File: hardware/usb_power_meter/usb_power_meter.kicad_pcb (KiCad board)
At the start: 4 copper layers, 33 x 24.6 mm, 30 parts, among them J1 Conn_ARM_JTAG_SWD_10, J2 USB_A, J4 USB_A, Q1 2N7002, Q2 IRML6401, U1 nRF52833-QDxx, U2 INA226, X1 32Mhz crystal, X2 32.768kHz crystal

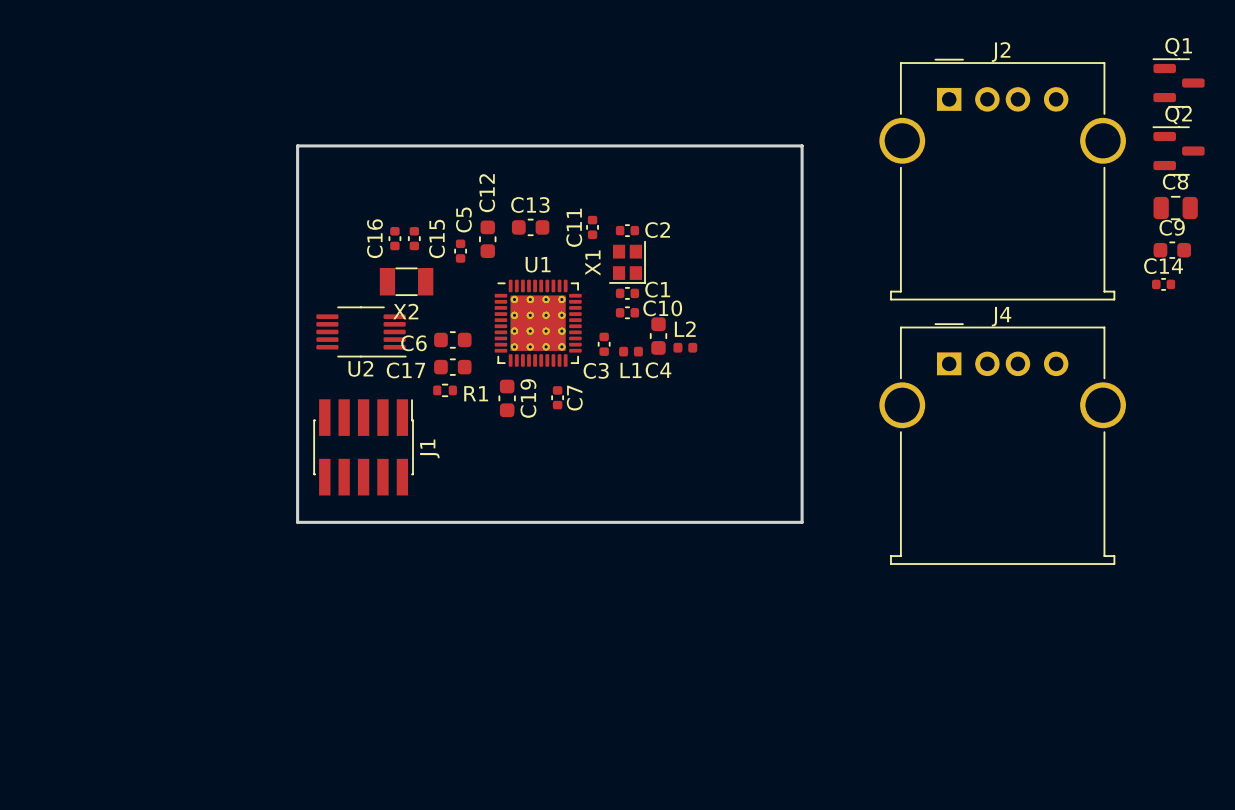
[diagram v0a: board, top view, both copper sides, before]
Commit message: Draft routing done
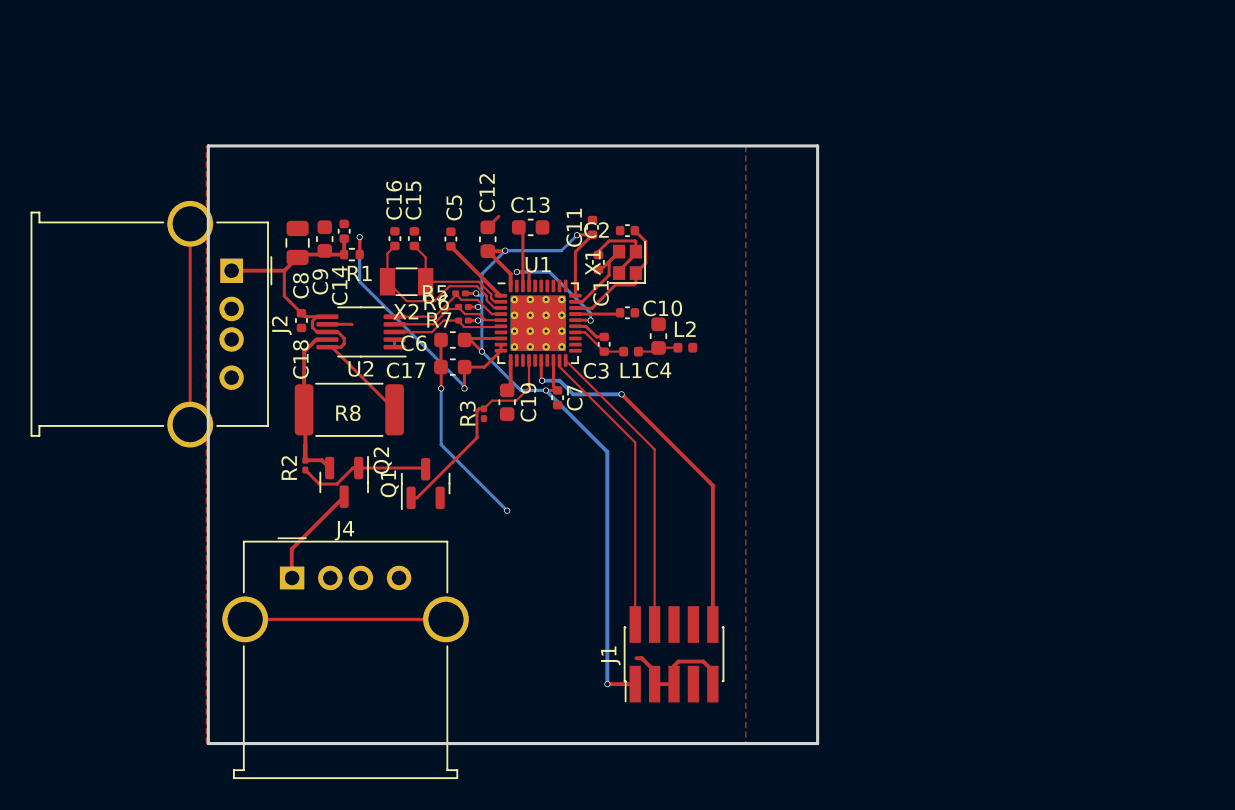
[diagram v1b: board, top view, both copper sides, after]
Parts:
- added C18: 100 nF, Capacitor_SMD:C_0402_1005Metric, F.Cu at (118.6, 102.6)
- added R2: 10k, Resistor_SMD:R_0201_0603Metric, F.Cu at (118.9, 112.1)
- added R3: 10k, Resistor_SMD:R_0201_0603Metric, F.Cu at (130.6, 108.7)
- added R5: 10k, Resistor_SMD:R_0201_0603Metric, F.Cu at (129.0, 100.8)
- added R6: 10k, Resistor_SMD:R_0201_0603Metric, F.Cu at (129.2, 101.7)
- added R7: 10k, Resistor_SMD:R_0201_0603Metric, F.Cu at (129.2, 102.6)
- added R8: LRP12FTDSR020, Resistor_SMD:R_2512_6332Metric, F.Cu at (121.8, 108.5)
- moved Q2 58.8 mm to (121.4, 113.2), turned to -90 degrees
- moved C8 57.5 mm to (118.4, 97.5), turned to 90 degrees
- moved Q1 55.8 mm to (126.7, 113.3), turned to 90 degrees
- moved C9 55.5 mm to (120.1, 97.3), turned to 90 degrees
- moved C14 53.7 mm to (121.4, 96.8), turned to 90 degrees
- moved J2 48.3 mm to (114.0, 99.4), turned to -90 degrees
- moved J4 45.2 mm to (118.0, 119.5)
- moved J1 24.4 mm to (143.0, 124.5), turned to 90 degrees
- moved R1 10.8 mm to (121.9, 98.3)
- moved C1 2.79 mm to (138.0, 98.8), turned to -90 degrees
- moved C5 1.01 mm to (128.4, 97.3)
- moved C19 0.25 mm to (132.1, 108.0)
- turned C2 to 0 degrees
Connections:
- Q2 pad 2: VBUS -> Net-(Q2-S)
- U2 pad 10: unconnected-(U2-Vin+-Pad10) -> VBUS
- U2 pad 9: unconnected-(U2-Vin--Pad9) -> Net-(Q2-S)
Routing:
- net VDD: track 0.00 -> 59.4 mm, vias 0 -> 8
- net GND: track 0.00 -> 35.5 mm, vias 0 -> 2
- net VBUS: track 0.00 -> 25.4 mm
- net Net-(J1-~{RESET}): track 0.00 -> 24.5 mm, vias 0 -> 2
- net Net-(J1-SWDCLK/TCK): track 0.00 -> 19.7 mm
- net Net-(J1-SWDIO/TMS): track 0.00 -> 19.3 mm
- net Net-(U1-VBUS): track 0.00 -> 18.8 mm, vias 0 -> 2
- net /EN_PWR: track 0.00 -> 14.0 mm
- net unconnected-(J2-Shield-Pad5): track 0.00 -> 13.1 mm
- net unconnected-(J4-Shield-Pad5): track 0.00 -> 13.1 mm
- net Net-(Q2-S): track 0.00 -> 11.8 mm
- net Net-(U1-DEC4): track 0.00 -> 11.8 mm, vias 0 -> 2
- net Net-(U1-XL2/P0.01): track 0.00 -> 11.6 mm
- net Net-(Q1-D): track 0.00 -> 8.72 mm
- net Net-(U1-XC1): track 0.00 -> 8.65 mm
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- added copper zone on F.Cu, net GND
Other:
- board size 33 x 24.6 mm -> 39.9 x 39.1 mm
